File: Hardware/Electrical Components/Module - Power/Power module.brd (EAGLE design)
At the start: 140 x 70 mm, 97 parts

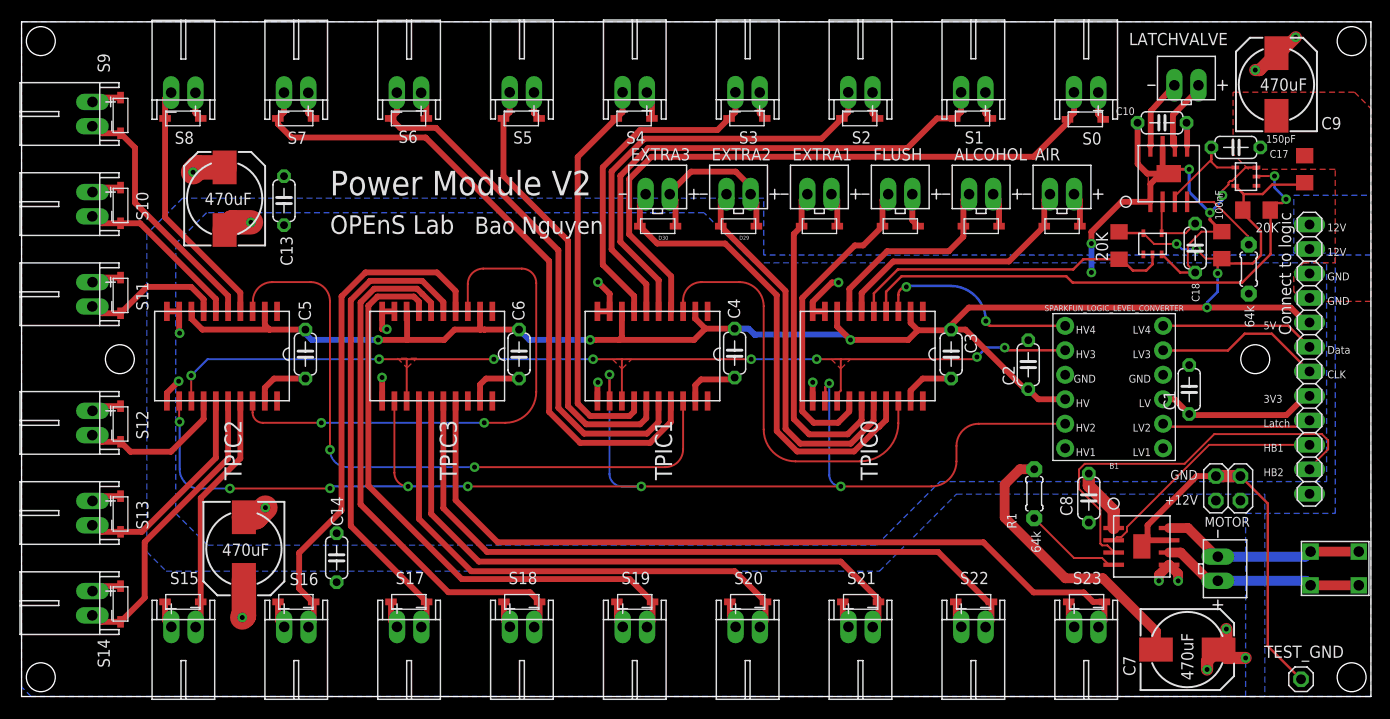
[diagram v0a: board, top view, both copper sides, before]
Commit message: Updates
Updated eDNA Eagle Library
Update OpenSPower7.2 BOM
Add OpenSPower 7.2 ReadMe
Add picture for FlowSensor
General clean up
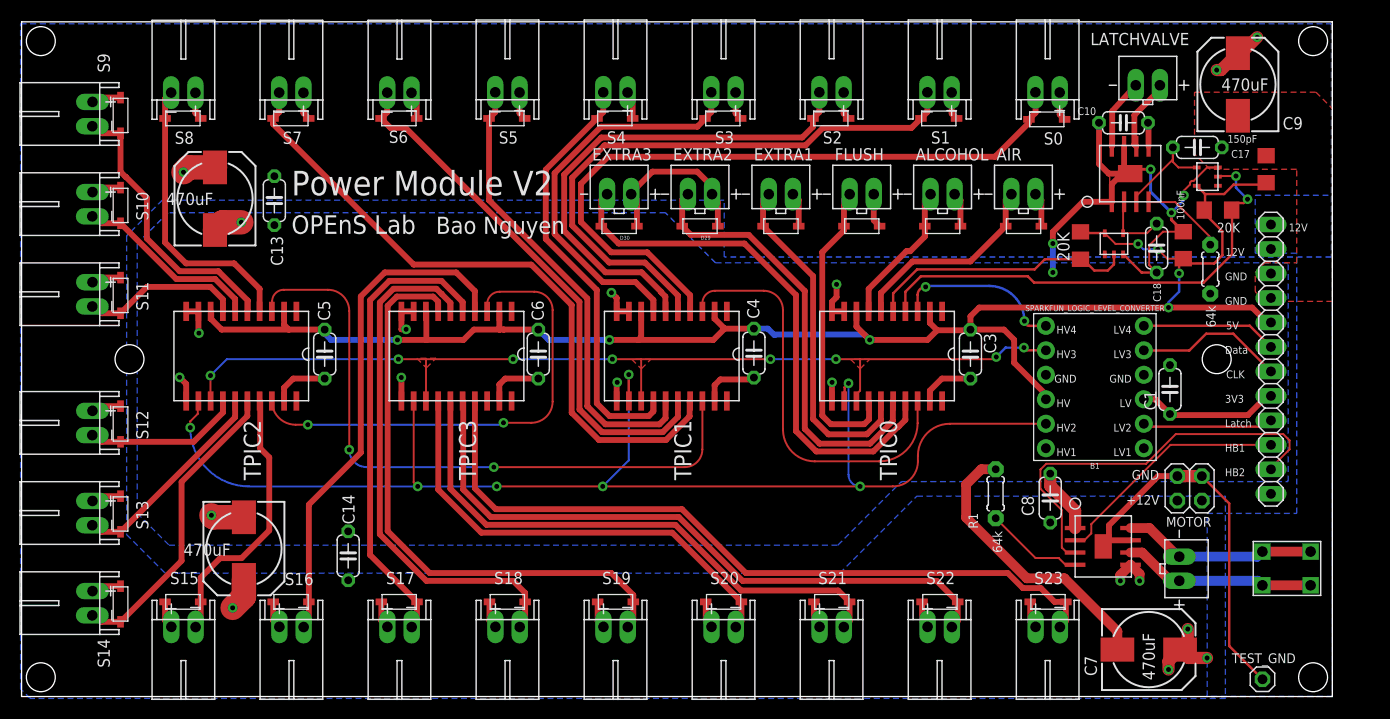
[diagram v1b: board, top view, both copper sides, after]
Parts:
- removed C2: 100nF, adafruit:C050-024X044
- moved U$1 5.00 mm to (131.1, 13.3)
- moved AIR 4.00 mm to (103.9, 52.1)
- moved ALCOHOL 4.00 mm to (95.6, 52.1)
- moved C10 4.00 mm to (114.3, 59.5)
- moved C11 4.00 mm to (120.5, 46.8)
- moved C12 4.00 mm to (129.1, 54.7)
- moved C17 4.00 mm to (122.0, 57.0)
- moved C18 4.00 mm to (117.8, 46.5)
- moved C7 4.00 mm to (117.0, 4.87)
- moved C8 4.00 mm to (106.7, 20.6)
- moved D1 4.00 mm to (106.4, 59.9)
- moved D24 4.00 mm to (106.5, 9.82)
- moved D25 4.00 mm to (104.0, 48.8)
- moved D26 4.00 mm to (95.6, 48.8)
- moved D27 4.00 mm to (87.2, 48.8)
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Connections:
- net +5V: no longer C2.1
- net GND: no longer C2.2
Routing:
- net T_RCK: track 143.1 -> 135.2 mm, vias 9 -> 7
- net +5V: track 192.4 -> 184.6 mm
- net S3: track 45.2 -> 52.5 mm
- net S4: track 34.5 -> 41.6 mm
- net S24: track 84.8 -> 78.1 mm
- net S22: track 64.9 -> 58.2 mm
- net S23: track 74.9 -> 68.2 mm
- net S2: track 55.9 -> 62.3 mm
- net S21: track 54.6 -> 48.3 mm
- net TPIC0_6: track 40.2 -> 46.2 mm
- net LATCHVALVE2: track 34.0 -> 28.0 mm
- net ALCOHOL: track 21.1 -> 15.1 mm
- net TPIC0_7: track 50.4 -> 56.4 mm
- net AIR: track 27.3 -> 21.3 mm
- net LATCHVALVE1: track 55.7 -> 49.7 mm
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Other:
- board size 140 x 70 mm -> 136 x 70 mm
